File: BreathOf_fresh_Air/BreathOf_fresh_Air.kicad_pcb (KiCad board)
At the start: 2 copper layers, 21.5 x 33 mm, 8 parts, among them J2 436500428, J3 436500227, U1 LM7805MPX/NOPB, U2 ALDP105W

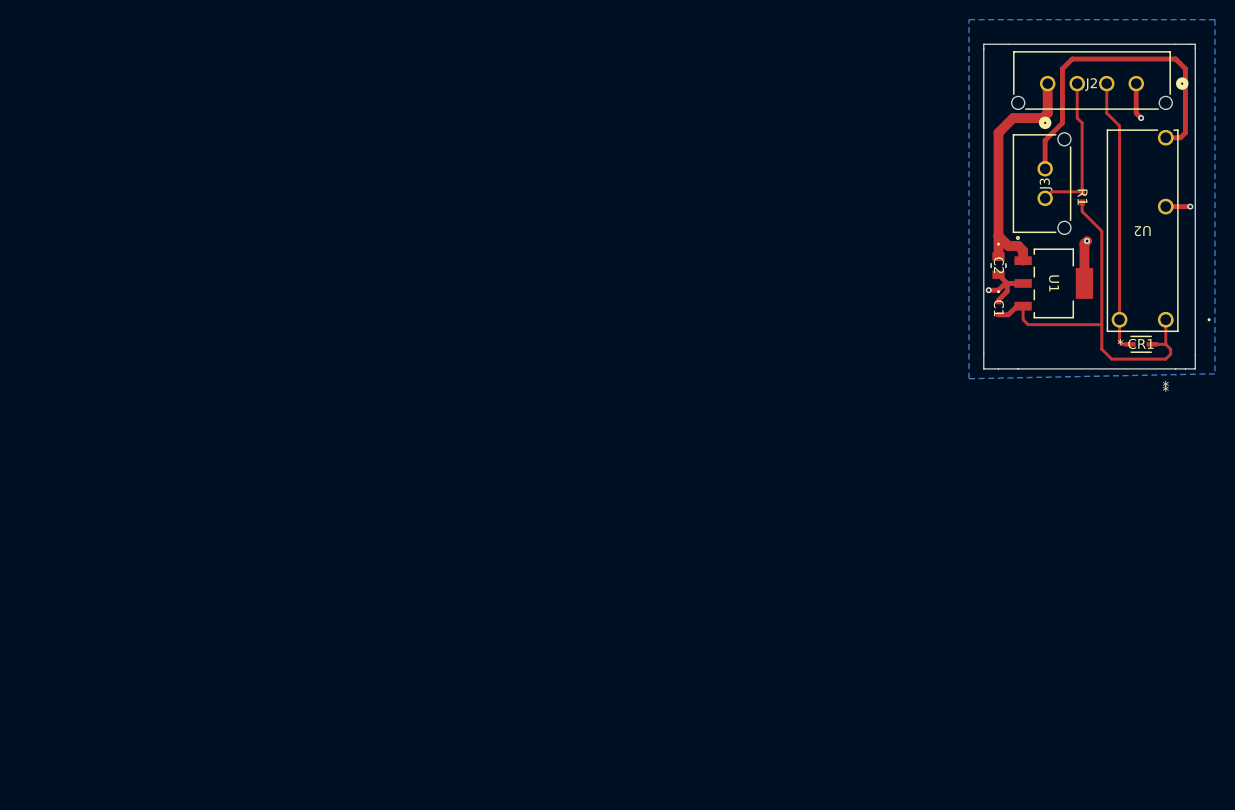
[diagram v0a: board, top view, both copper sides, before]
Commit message: updated
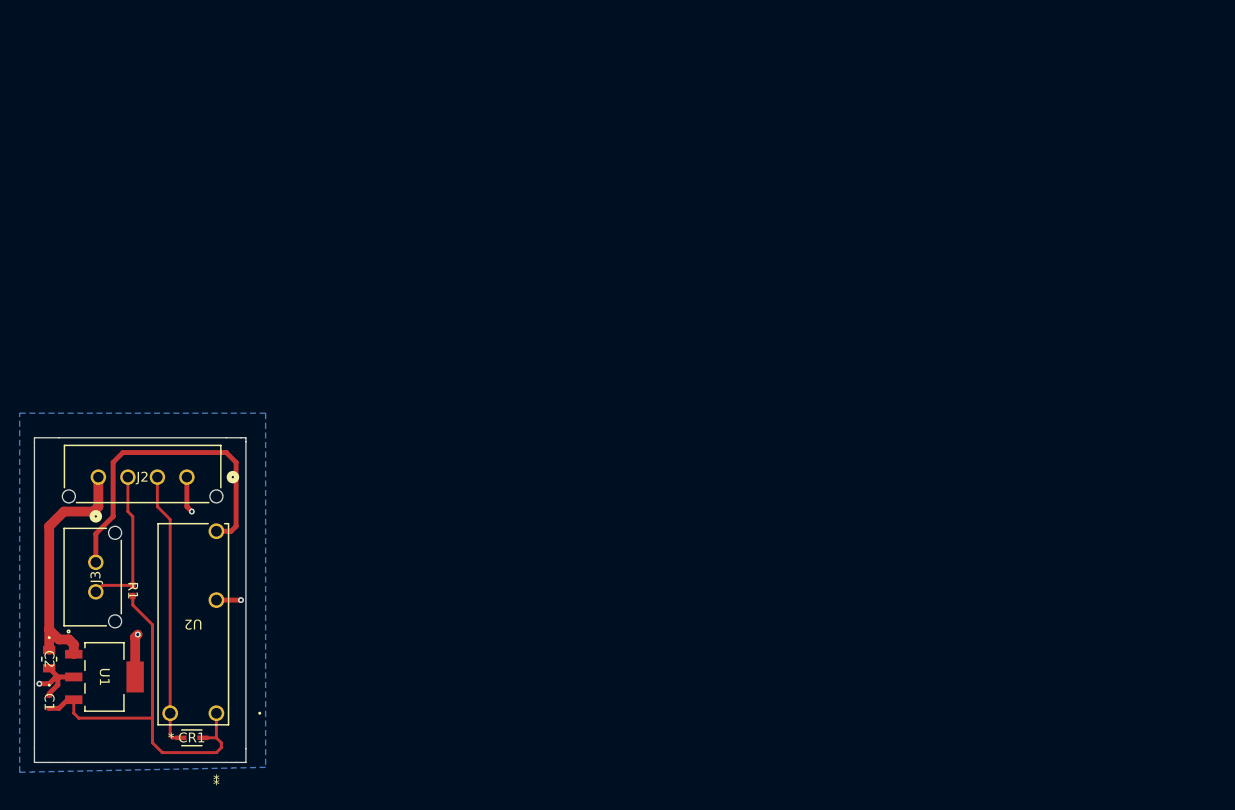
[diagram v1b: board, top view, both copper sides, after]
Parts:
- moved C1 104.5 mm to (131.5, 105.9)
- moved C2 104.5 mm to (131.5, 101.5)
- moved CR1 104.5 mm to (146.0, 109.5)
- moved J2 104.5 mm to (145.5, 83.0)
- moved J3 104.5 mm to (136.2, 91.7)
- moved R1 104.5 mm to (140.0, 94.5)
- moved U1 104.5 mm to (137.1, 103.3)
- moved U2 104.5 mm to (148.5, 107.0)
